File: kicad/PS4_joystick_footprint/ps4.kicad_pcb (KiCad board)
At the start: 2 copper layers, 20 x 28.5 mm, 2 parts, among them J1 Joystick, U1 COM-09032

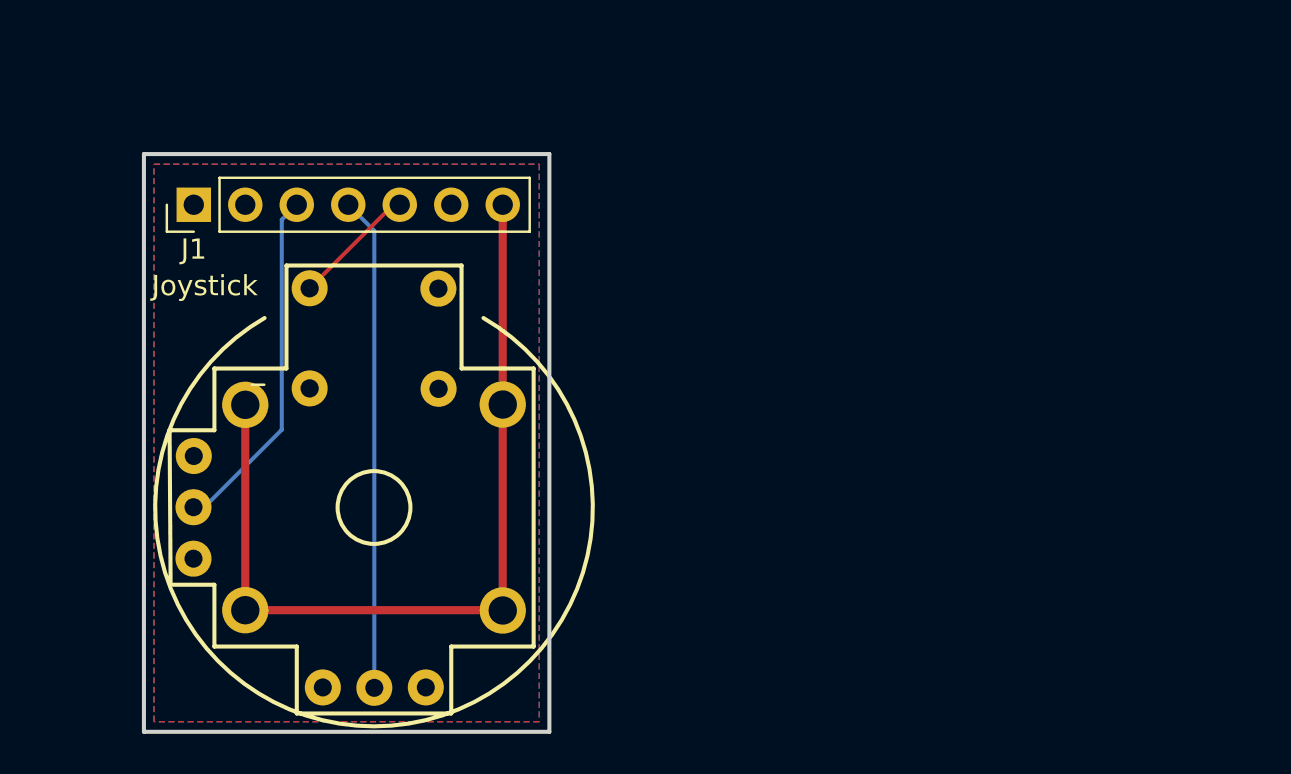
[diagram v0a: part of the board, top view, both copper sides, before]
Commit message: update pcb and documentation
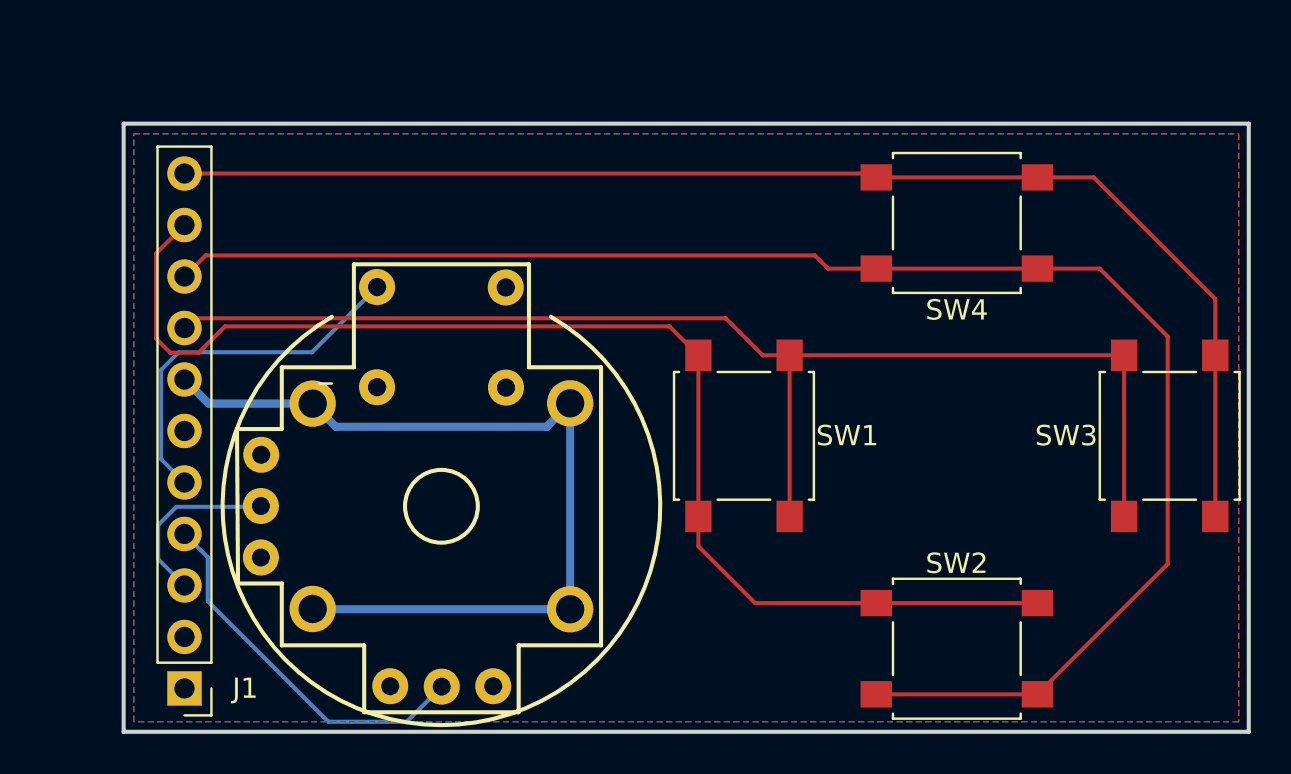
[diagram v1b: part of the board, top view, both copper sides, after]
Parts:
- added SW1: SW_Push, Button_Switch_SMD:SW_SPST_B3S-1000, F.Cu at (119.5, 140.5)
- added SW2: SW_Push, Button_Switch_SMD:SW_SPST_B3S-1000, F.Cu at (130.0, 151.0)
- added SW3: SW_Push, Button_Switch_SMD:SW_SPST_B3S-1000, F.Cu at (140.5, 140.5)
- added SW4: SW_Push, Button_Switch_SMD:SW_SPST_B3S-1000, F.Cu at (130.0, 130.0)
- J1: value Joystick -> Conn_01x11_Pin; footprint Connector_PinHeader_2.54mm:PinHeader_1x07_P2.54mm_Vertical -> Connector_PinHeader_2.54mm:PinHeader_1x11_P2.54mm_Vertical
- moved J1 23.9 mm to (91.9, 153.0), turned to 180 degrees
- moved U1 3.33 mm to (104.6, 144.0)
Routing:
- net /L2: track 0.00 -> 78.9 mm
- net /R2: track 0.00 -> 64.1 mm
- net /L1: track 0.00 -> 63.2 mm
- net /R1: track 0.00 -> 61.7 mm
- net /Switch: track 6.15 -> 18.4 mm
- net /R_black: track 17.3 -> 9.50 mm
- net /R_orange: track 24.4 -> 18.5 mm
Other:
- board size 20 x 28.5 mm -> 55.5 x 30 mm
